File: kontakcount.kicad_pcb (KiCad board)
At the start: 4 copper layers, 55 x 100 mm, 49 parts

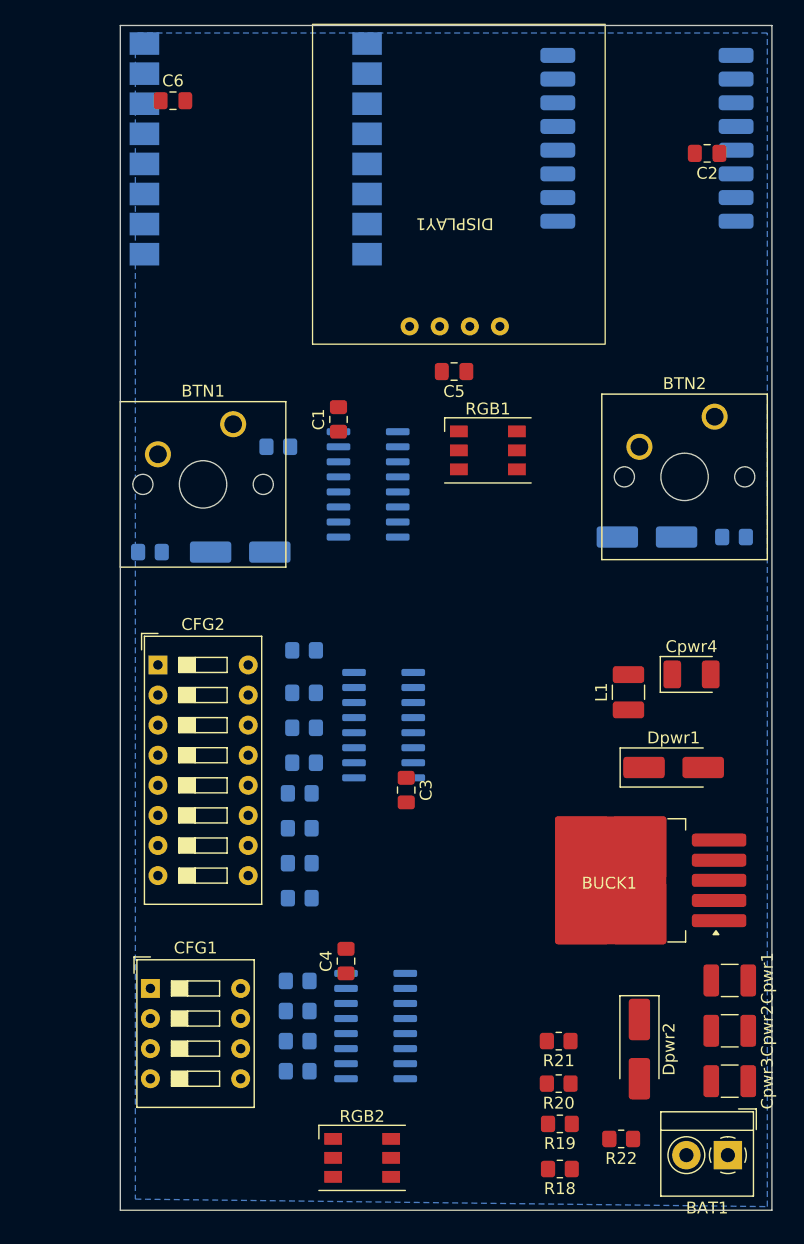
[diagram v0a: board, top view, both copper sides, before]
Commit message: routing progress towards v001
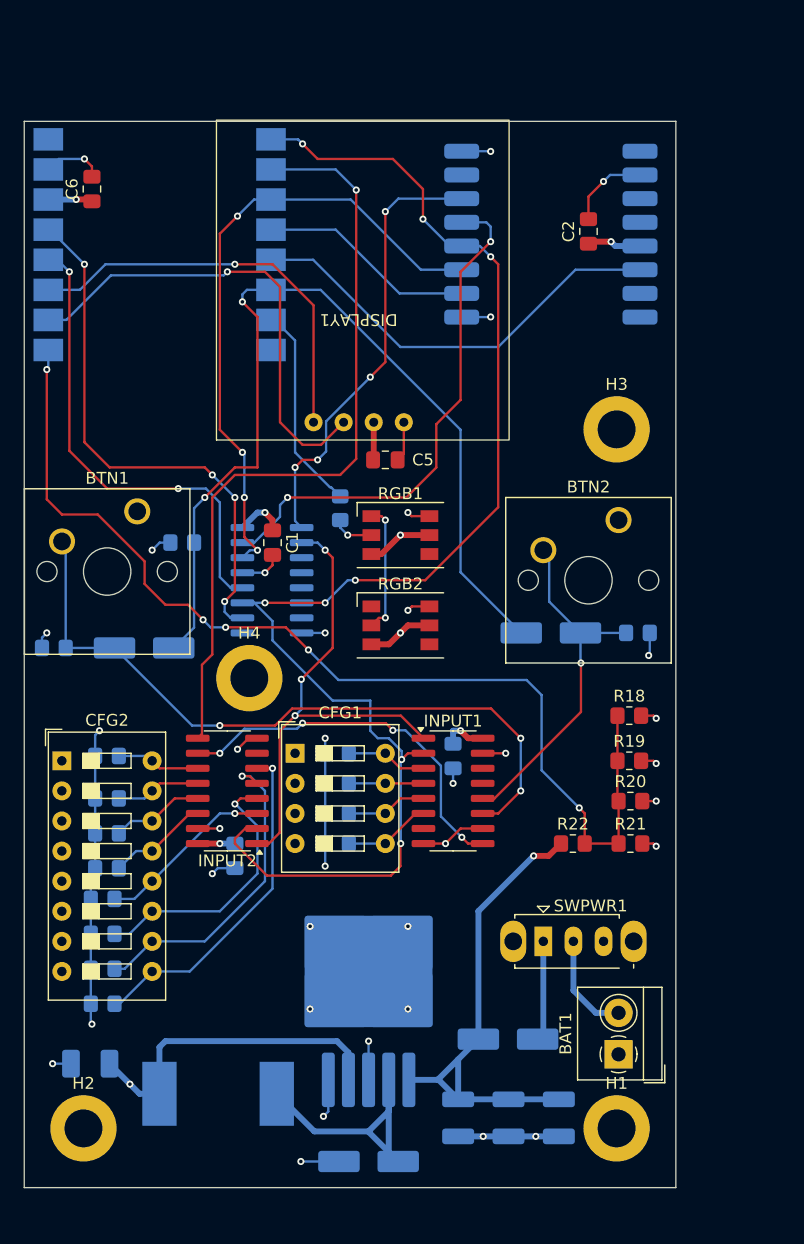
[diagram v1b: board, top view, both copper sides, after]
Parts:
- added H1: MountingHole_Pad, MountingHole:MountingHole_3.2mm_M3_DIN965_Pad, F.Cu at (160.0, 135.0)
- added H2: MountingHole_Pad, MountingHole:MountingHole_3.2mm_M3_DIN965_Pad, F.Cu at (115.0, 135.0)
- added H3: MountingHole_Pad, MountingHole:MountingHole_3.2mm_M3_DIN965_Pad, F.Cu at (160.0, 76.0)
- added H4: MountingHole_Pad, MountingHole:MountingHole_3.2mm_M3_DIN965_Pad, F.Cu at (129.0, 97.0)
- added R23: 0, Resistor_SMD:R_0805_2012Metric_Pad1.20x1.40mm_HandSolder, B.Cu at (136.7, 82.7)
- added SWPWR1: SW_SPDT, xandy1:POWERSWITCH SLIDE THT, F.Cu at (153.8, 119.2)
- BUCK1, C3, C4, Cpwr1, Cpwr2, Cpwr3, Cpwr4, Dpwr1, Dpwr2: moved to B.Cu
- INPUT1, INPUT2: moved to F.Cu
- L1: footprint Inductor_SMD:L_1210_3225Metric_Pad1.42x2.65mm_HandSolder -> Inductor_SMD:L_12x12mm_H6mm; moved to B.Cu
- moved Cpwr4 60.5 mm to (115.6, 129.5), turned to 180 degrees
- moved L1 48.5 mm to (126.4, 132.1), turned to 180 degrees
- moved RGB2 45.1 mm to (141.8, 92.5)
- moved Dpwr1 42.1 mm to (139.1, 137.8), turned to 180 degrees
- moved R18 38.7 mm to (161.1, 100.2), turned to 0 degrees
- moved R19 31.2 mm to (161.1, 104.0), turned to 0 degrees
- moved Cpwr1 25.7 mm to (146.6, 134.1), turned to -90 degrees
- moved R22 25.3 mm to (156.3, 111.0), turned to 0 degrees
- moved R20 24.6 mm to (161.2, 107.4), turned to 0 degrees
- moved BUCK1 23.8 mm to (139.1, 123.3), turned to 90 degrees
- moved CFG1 23.3 mm to (132.9, 103.3)
- moved INPUT1 20.9 mm to (146.2, 106.5), turned to 0 degrees
- moved Cpwr2 20.1 mm to (150.9, 134.1), turned to -90 degrees
- moved C4 19.5 mm to (146.2, 103.6), turned to -90 degrees
- moved R8 19.5 mm to (136.4, 111.0), turned to 180 degrees
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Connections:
- BAT1 pad 2: /Power/VBATT -> Net-(BAT1-Pin_2)
- BUCK1 pad 1: Net-(BUCK1-VIN) -> /Power/VBATT
- Cpwr1 pad 1: Net-(BUCK1-VIN) -> /Power/VBATT
- Cpwr2 pad 1: Net-(BUCK1-VIN) -> /Power/VBATT
- Cpwr3 pad 1: Net-(BUCK1-VIN) -> /Power/VBATT
- Dpwr2 pad 1: Net-(BUCK1-VIN) -> /Power/VBATT
- Dpwr2 pad 2: /Power/VBATT -> Net-(Dpwr2-A)
- ESP32-C3 pad 5: Net-(CHSEL1-SER) -> /CLK
- ESP32-C3 pad 7: Net-(ESP32-C3-GPIO7) -> Net-(CHSEL1-SER)
- LORA1 pad 3: Net-(ESP32-C3-GPIO7) -> Net-(CHSEL1-SER)
- RGB1 pad 2: Net-(ESP32-C3-GPIO20) -> Net-(RGB1-DIN)
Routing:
- net /CLK: track 0.00 -> 120.3 mm, vias 0 -> 8
- net GND: track 0.00 -> 109.6 mm, vias 0 -> 35
- net Net-(ESP32-C3-GPIO0): track 0.00 -> 90.0 mm, vias 0 -> 5
- net /INPUT_INT: track 0.00 -> 77.1 mm, vias 0 -> 2
- net /Input/DO: track 0.00 -> 64.9 mm, vias 0 -> 1
- net VCC: track 0.00 -> 61.4 mm, vias 0 -> 8
- net Net-(ID1-A): track 0.00 -> 59.1 mm, vias 0 -> 3
- net Net-(CHSEL1-SER): track 0.00 -> 53.6 mm, vias 0 -> 4
- net Net-(CHSEL1-~{SRCLR}): track 0.00 -> 45.5 mm, vias 0 -> 4
- net Net-(CHSEL1-QA): track 0.00 -> 44.4 mm, vias 0 -> 2
- net /Input/~{PL}: track 0.00 -> 42.1 mm, vias 0 -> 3
- net /Power/VBATT: track 0.00 -> 41.7 mm, vias 0 -> 1
- net Net-(DISPLAY1-SCL): track 0.00 -> 40.1 mm, vias 0 -> 1
- net Net-(CHSEL1-RCLK): track 0.00 -> 39.6 mm, vias 0 -> 2
- net Net-(CHSEL1-QB): track 0.00 -> 37.7 mm, vias 0 -> 4
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- added copper zone on In2.Cu, net GND
- removed copper zone on B.Cu, net GND
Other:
- board size 55 x 100 mm -> 55 x 90 mm
